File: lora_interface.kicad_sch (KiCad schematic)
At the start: 2 parts, among them J6 SMA

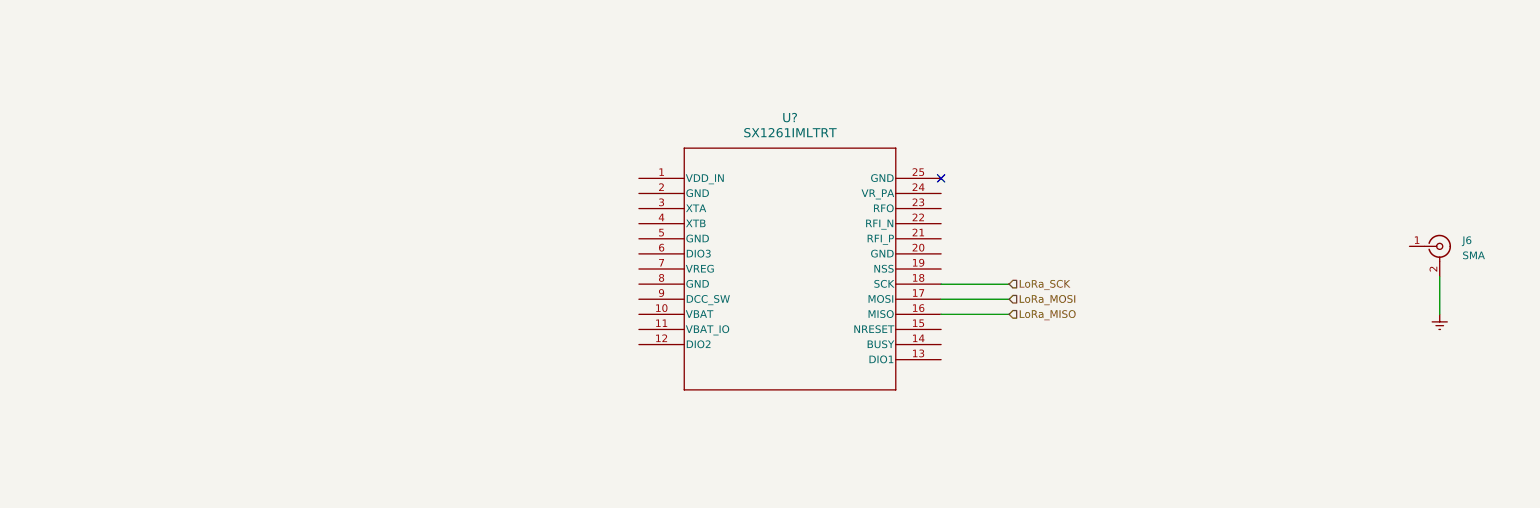
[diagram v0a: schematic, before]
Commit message: version 1
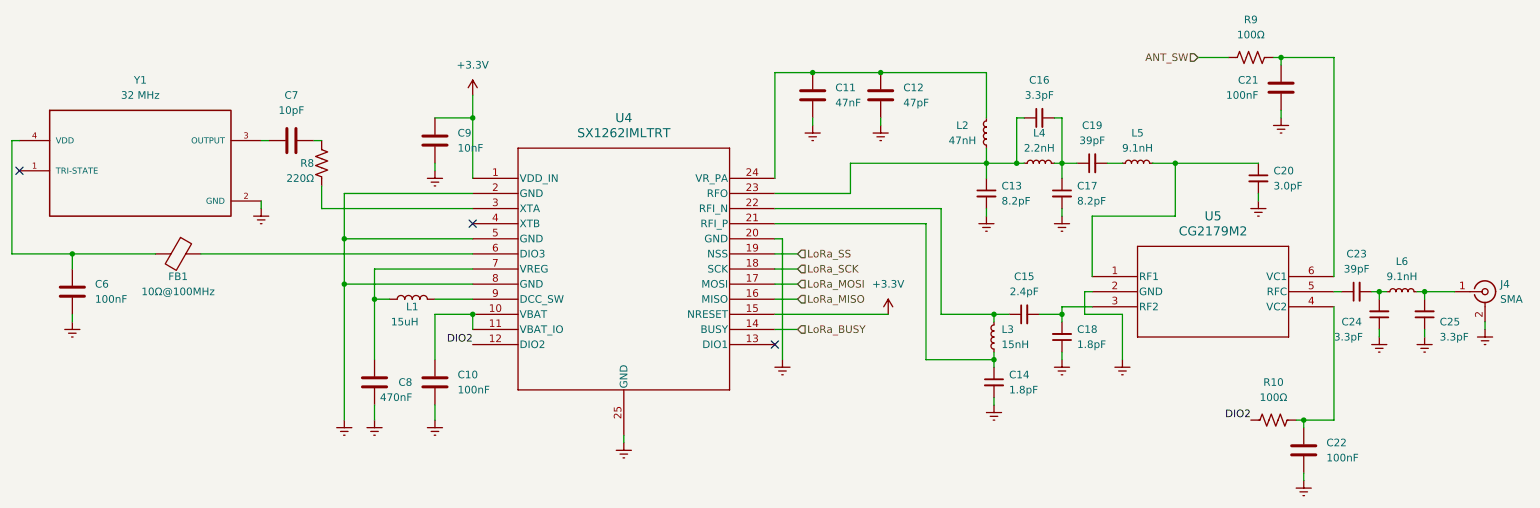
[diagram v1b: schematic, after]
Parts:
- removed U?: SX1261IMLTRT, QFN4x4_SEM, symbol SX1261:SX1261IMLTRT
- added C10, C6: 100nF, Capacitor_SMD:C_0402_1005Metric_Pad0.74x0.62mm_HandSolder, symbol Device:C
- added C11: 47nF, Capacitor_SMD:C_0402_1005Metric_Pad0.74x0.62mm_HandSolder, symbol Device:C
- added C12: 47pF, Capacitor_SMD:C_0402_1005Metric_Pad0.74x0.62mm_HandSolder, symbol Device:C
- added C13, C17: 8.2pF, Capacitor_SMD:C_0402_1005Metric_Pad0.74x0.62mm_HandSolder, symbol Device:C_Small
- added C14, C18: 1.8pF, Capacitor_SMD:C_0402_1005Metric_Pad0.74x0.62mm_HandSolder, symbol Device:C_Small
- added C15: 2.4pF, Capacitor_SMD:C_0402_1005Metric_Pad0.74x0.62mm_HandSolder, symbol Device:C_Small
- added C16, C24, C25: 3.3pF, Capacitor_SMD:C_0402_1005Metric_Pad0.74x0.62mm_HandSolder, symbol Device:C_Small
- added C19, C23: 39pF, Capacitor_SMD:C_0402_1005Metric_Pad0.74x0.62mm_HandSolder, symbol Device:C_Small
- added C20: 3.0pF, Capacitor_SMD:C_0402_1005Metric_Pad0.74x0.62mm_HandSolder, symbol Device:C_Small
- added C21, C22: 100nF, Capacitor_SMD:C_0805_2012Metric_Pad1.18x1.45mm_HandSolder, symbol Device:C
- added C7: 10pF, Capacitor_SMD:C_0402_1005Metric_Pad0.74x0.62mm_HandSolder, symbol Device:C
- added C8: 470nF, Capacitor_SMD:C_0402_1005Metric_Pad0.74x0.62mm_HandSolder, symbol Device:C
- added C9: 10nF, Capacitor_SMD:C_0402_1005Metric_Pad0.74x0.62mm_HandSolder, symbol Device:C
- added FB1: 10Ω@100MHz, Inductor_SMD:L_0402_1005Metric_Pad0.77x0.64mm_HandSolder, symbol Device:FerriteBead
- added L1: 15uH, Inductor_SMD:L_0402_1005Metric_Pad0.77x0.64mm_HandSolder, symbol Device:L
- added L2: 47nH, Inductor_SMD:L_0402_1005Metric_Pad0.77x0.64mm_HandSolder, symbol Device:L_Small
- added L3: 15nH, Inductor_SMD:L_0402_1005Metric_Pad0.77x0.64mm_HandSolder, symbol Device:L_Small
- added L4: 2.2nH, Inductor_SMD:L_0402_1005Metric_Pad0.77x0.64mm_HandSolder, symbol Device:L_Small
- added L5, L6: 9.1nH, Inductor_SMD:L_0402_1005Metric_Pad0.77x0.64mm_HandSolder, symbol Device:L_Small
- added R10, R9: 100Ω, Resistor_SMD:R_0805_2012Metric_Pad1.20x1.40mm_HandSolder, symbol Device:R_US
- added R8: 220Ω, Resistor_SMD:R_0402_1005Metric_Pad0.72x0.64mm_HandSolder, symbol Device:R_US
- added U4: SX1262IMLTRT, Library:QFN24_4X4_SEM, symbol SX1262:SX1262IMLTRT
- added U5: CG2179M2, Library:MINISO6_CG21_CEL, symbol rfswitch:CG2179M2
- added Y1: 32 MHz, Library:OSC_ECS-TXO-2520-33-320-AN-TR, symbol TCXO:ECS-TXO-2520-33-320-AN-TR
- J4: renamed from J6; footprint (none) -> Connector_Coaxial:SMA_Samtec_SMA-J-P-X-ST-EM1_EdgeMount
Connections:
- net GNDREF: now also C10.2, C11.2, C12.2, C13.2, C14.2, C17.2, C18.1, C20.2, C21.2, C22.2, C24.1, C25.1, C6.2, C8.2, C9.2, U4.2 (GND), U4.20 (GND), U4.25 (GND), U4.5 (GND), U4.8 (GND), U5.2 (GND), Y1.2 (GND)
- net LoRa_MISO: now also U4.16 (MISO)
- net LoRa_MOSI: now also U4.17 (MOSI)
- net LoRa_SCK: now also U4.18 (SCK)
- net at J4.1 (In): now also C25.2, L6.2
- new net: C14.1, L3.1, U4.21 (RFI_P)
- new net: C23.2, C24.2, L6.1
- new net: C16.2, C17.1, C19.1, L4.2
- new net: C13.1, C16.1, L2.1, L4.1, U4.23 (RFO)
- new net: C10.1, U4.10 (VBAT), U4.11 (VBAT_IO)
- new net: C15.1, L3.2, U4.22 (RFI_N)
- new net: C11.1, C12.1, L2.2, U4.24 (VR_PA)
- new net: R8.2, U4.3 (XTA)
- new net: FB1.1, U4.6 (DIO3)
- new net: C8.1, L1.1, U4.7 (VREG)
- new net: L1.2, U4.9 (DCC_SW)
- new net: C7.1, Y1.3 (OUTPUT)
- new net: C7.2, R8.1
- new net: C23.1, U5.5 (RFC)
- new net: C21.1, R9.2, U5.6 (VC1)
- new net: C20.1, L5.2, U5.1 (RF1)
- new net: C15.2, C18.2, U5.3 (RF2)
- new net: C6.1, FB1.2, Y1.4 (VDD)
- new net: C19.2, L5.1
- new net: C22.1, R10.2, U5.4 (VC2)
- new net +3.3V: C9.1, U4.1 (VDD_IN), U4.15 (NRESET)
- new net ANT_SW: R9.1
- new net DIO2: R10.1, U4.12 (DIO2)
- new net LoRa_BUSY: U4.14 (BUSY)
- new net LoRa_SS: U4.19 (NSS)
- no-connect marks 1 -> 3
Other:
- company: (none) -> Texas A&M ECEN Capstone
- title: (none) -> LoRa Interface
- moved on the sheet: J4
